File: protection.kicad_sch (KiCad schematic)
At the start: 25 parts, among them J4 Conn_01x04, Q2 NMOS, Q3 NMOS, Q4 NMOS

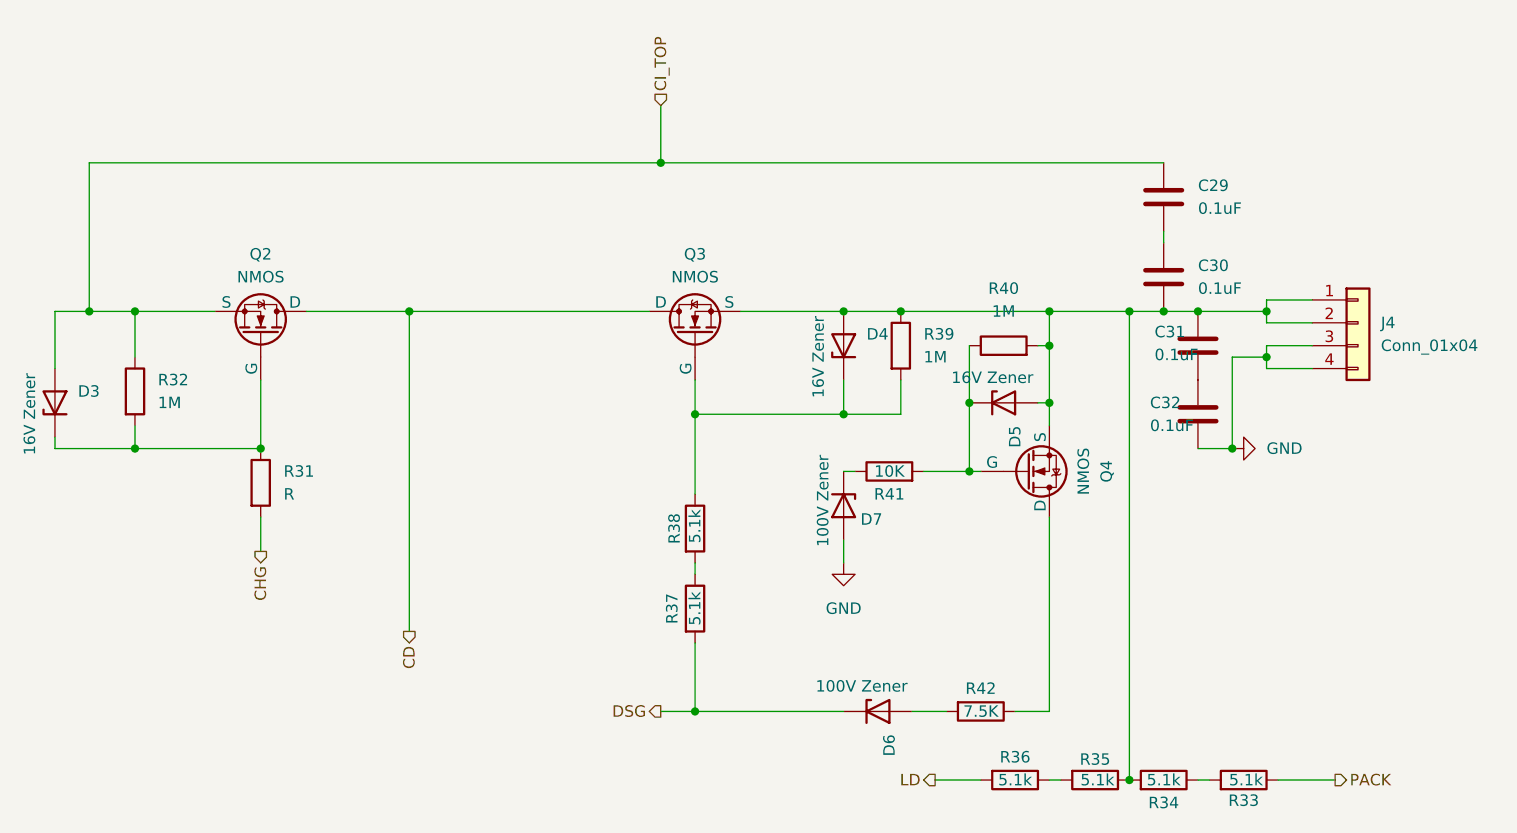
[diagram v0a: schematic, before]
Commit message: lots of lots changes. Schematic done NEEDS Review
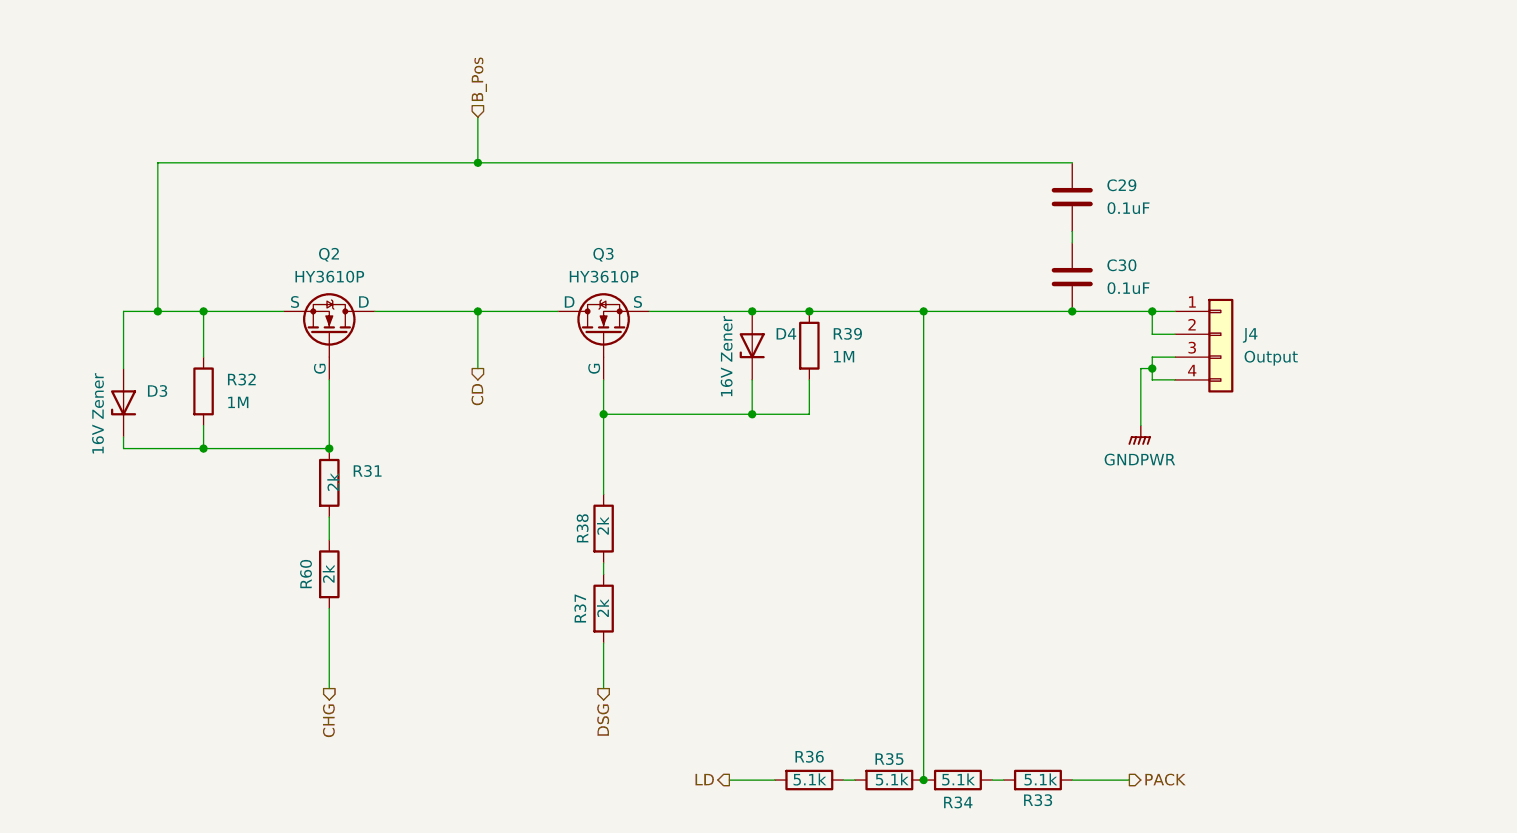
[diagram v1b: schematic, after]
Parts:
- removed C31, C32: 0.1uF, symbol Device:C
- removed D5: 16V Zener, symbol Device:D_Zener
- removed D6, D7: 100V Zener, symbol Device:D_Zener
- removed Q4: NMOS, Package_TO_SOT_THT:TO-220-3_Vertical, symbol Simulation_SPICE:NMOS
- removed R40: 1M, symbol Device:R
- removed R41: 10K, symbol Device:R
- removed R42: 7.5K, symbol Device:R
- added R60: 2k, symbol Device:R
- J4: value Conn_01x04 -> Output
- Q2, Q3: value NMOS -> HY3610P
- R31: value R -> 2k
- R37, R38: value 5.1k -> 2k
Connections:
- net CHG: now also R60.2; no longer R31.2
- net CI_TOP renamed B_Pos
- net GND renamed GNDPWR
- new net: R31.2, R60.1
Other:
- company: (none) -> Pehlivan Team
- title: (none) -> Pehli-Shell-BMS
- moved on the sheet: C29, C30, D3, D4, Q2, Q3, R31, R32, R33, R34, R35, R36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
